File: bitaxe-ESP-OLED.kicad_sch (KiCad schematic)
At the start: 48 parts, among them J1 SFV30R-4STE1HLF, J2 Conn_01x06, J3 USB_C_Receptacle_USB2.0_16P, Q1 SI2307, SW1 SWITCH-SPST, SW2 SWITCH-SPST, SW3 SWITCH-SPST, SW4 SWITCH-SPST, U1 ESP32_S3R8, U2 RT9080-33GJ5, U3 AP2502KTR-G1, U4 W25Q128JV, Y2 40 MHz

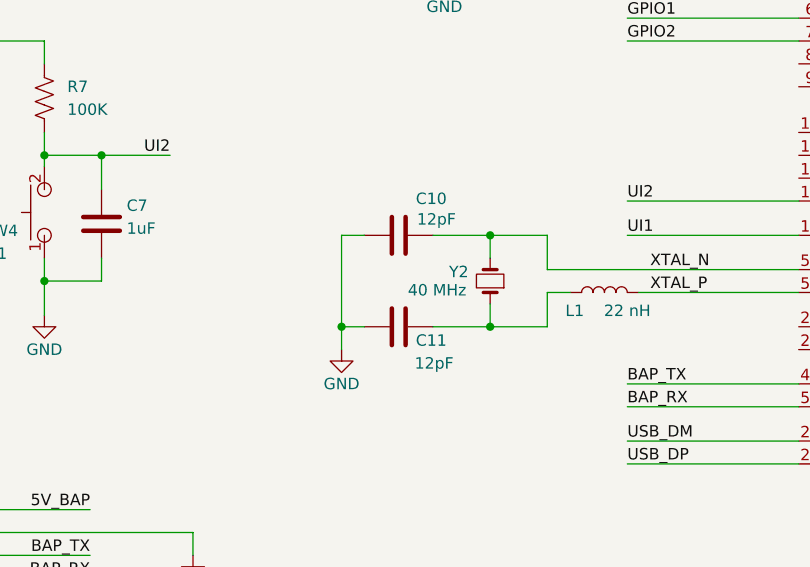
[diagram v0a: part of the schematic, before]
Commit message: Finish up routing
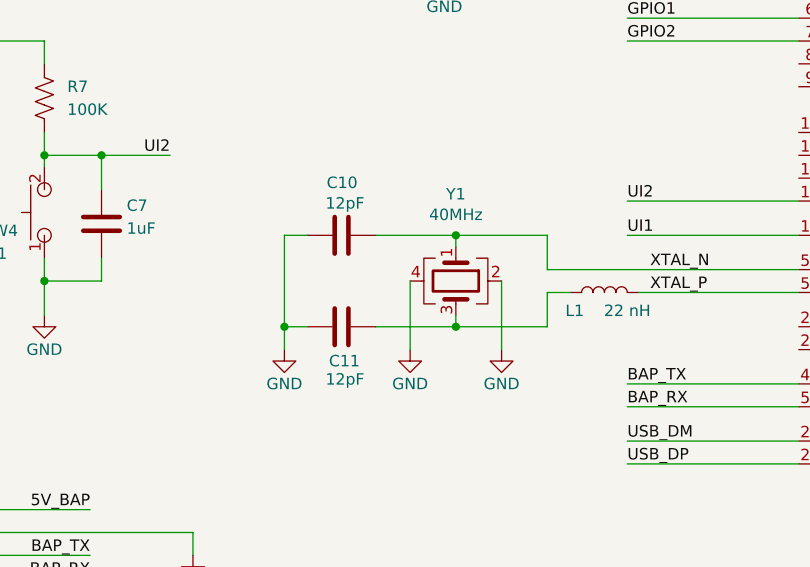
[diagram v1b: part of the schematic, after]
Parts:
- removed Y2: 40 MHz, bitaxe:Abracon-ABM3, symbol Device:Crystal_Small
- added Y1: 40MHz, bitaxe:RH100-oscillator, symbol Device:Crystal_GND24
- U1: footprint Package_DFN_QFN:QFN-56-1EP_7x7mm_P0.4mm_EP4x4mm_ThermalVias -> bitaxe:QFN-56-1EP_7x7mm_P0.4mm_EP4x4mm_ThermalVias
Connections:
- net GND: now also Y1.2, Y1.4
- net XTAL_N: now also Y1.1
- net at C11.2, L1.1: now also Y1.3
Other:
- moved on the sheet: C10, C11
